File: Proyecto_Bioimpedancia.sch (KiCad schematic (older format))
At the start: 69 parts, among them J1 Jumper, J2 Jumper, J3 Jumper_Calibration, J4 Jumper, J5 Jumper, J6 Jumper, P1 SD_LAPIZ, P10 RS-232, P11 SOURCE_2, P12 RESET, P13 POWER, P14 BIO_OUT1, P15 GND_REGULATOR, P16 BIO_OUT2, P2 GPIO, P3 SOURCE_3, P4 SERIAL_VIRTUAL, P5 ENCODER, P6 I2C_1, P7 I2C_2, P8 SOURCE_1, P9 SPI, SW1 SW_PUSH, U1 AD8606, U2 ADG819, U3 Atmega328PA, U4 LD1117S50TR, Y1 XRCHA_16M

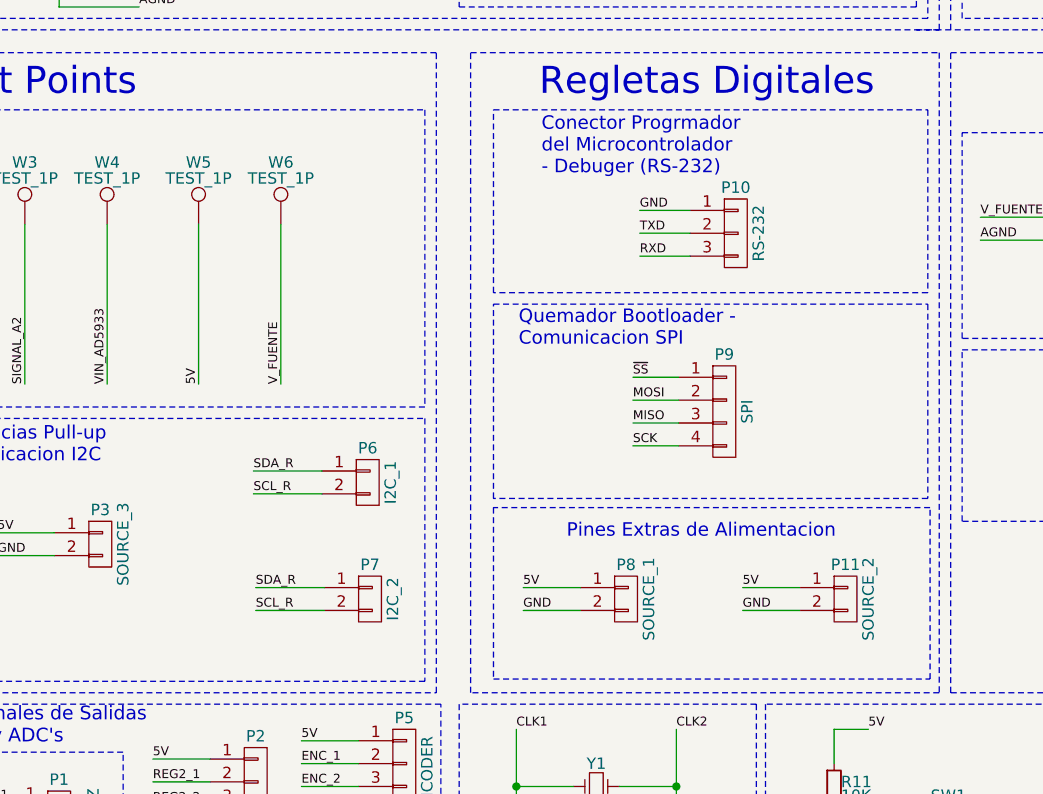
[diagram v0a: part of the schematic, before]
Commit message: PCB BIO mejorada con puertos I2C y capacitor para el puerto DTR del programador FTDI
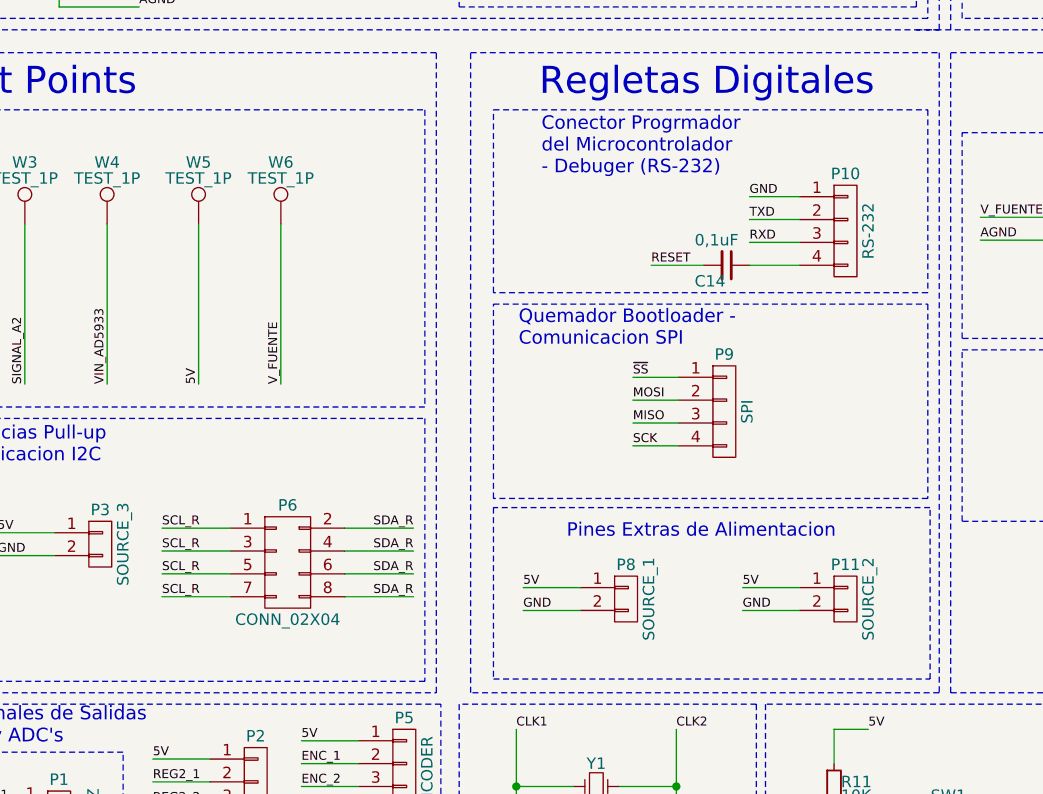
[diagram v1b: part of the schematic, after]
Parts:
- removed P10: RS-232, Socket_Strips:Socket_Strip_Straight_1x03_Pitch2.54mm, symbol CONN_01X03
- removed P6: I2C_1, Socket_Strips:Socket_Strip_Straight_1x02_Pitch2.54mm, symbol CONN_01X02
- removed P7: I2C_2, Socket_Strips:Socket_Strip_Straight_1x02_Pitch2.54mm, symbol CONN_01X02
- added C14: 0,1uF, Capacitors_SMD:C_0805_HandSoldering, symbol 0,1uF
- added P10: RS-232, Socket_Strips:Socket_Strip_Straight_1x04_Pitch2.54mm, symbol CONN_01X04
- added P6: CONN_02X04, Socket_Strips:Socket_Strip_Straight_2x04_Pitch2.54mm, symbol CONN_02X04
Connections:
- net AGND: now also P10.1 (P1)
- net RESET: now also C14.2
- net RXD: now also P10.3 (P3)
- net SCL_R: now also P6.1 (P1), P6.3 (P3), P6.5 (P5), P6.7 (P7)
- net SDA_R: now also P6.2 (P2), P6.4 (P4), P6.6 (P6), P6.8 (P8)
- net TXD: now also P10.2 (P2)
- new net: C14.1, P10.4 (P4)

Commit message: Revert "PCB BIO mejorada con puertos I2C y capacitor para el puerto DTR del programador FTDI"
This reverts commit 0fb084b6cb4dcbd826a5771fbeb8258d6327cef0.
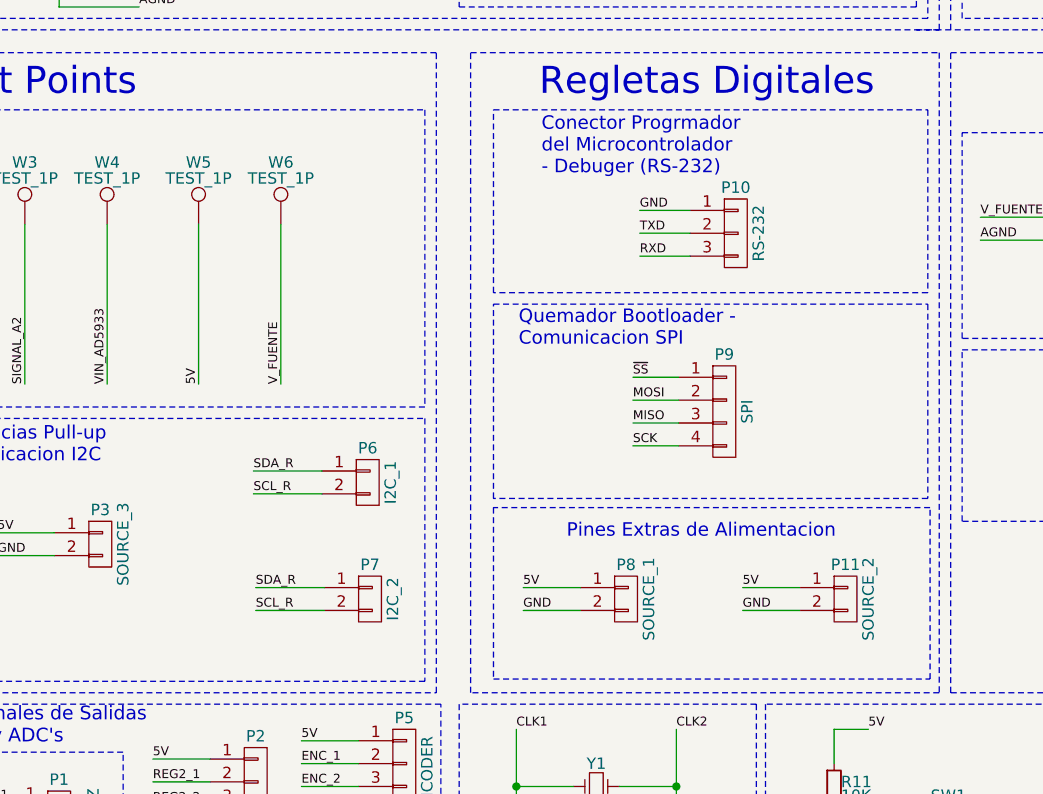
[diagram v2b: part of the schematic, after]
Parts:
- removed C14: 0,1uF, Capacitors_SMD:C_0805_HandSoldering, symbol 0,1uF
- removed P10: RS-232, Socket_Strips:Socket_Strip_Straight_1x04_Pitch2.54mm, symbol CONN_01X04
- removed P6: CONN_02X04, Socket_Strips:Socket_Strip_Straight_2x04_Pitch2.54mm, symbol CONN_02X04
- added P10: RS-232, Socket_Strips:Socket_Strip_Straight_1x03_Pitch2.54mm, symbol CONN_01X03
- added P6: I2C_1, Socket_Strips:Socket_Strip_Straight_1x02_Pitch2.54mm, symbol CONN_01X02
- added P7: I2C_2, Socket_Strips:Socket_Strip_Straight_1x02_Pitch2.54mm, symbol CONN_01X02
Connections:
- net AGND: now also P10.1 (P1)
- net RXD: now also P10.3 (P3)
- net SCL_R: now also P6.2 (P2), P7.2 (P2)
- net SDA_R: now also P6.1 (P1), P7.1 (P1)
- net TXD: now also P10.2 (P2)
